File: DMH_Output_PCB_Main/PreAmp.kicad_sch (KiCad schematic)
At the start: 39 parts, among them J13 Conn_01x06, J28 Conn_01x06, U16 NE5532, U17 NE5532, U18 NE5532, U19 NE5532

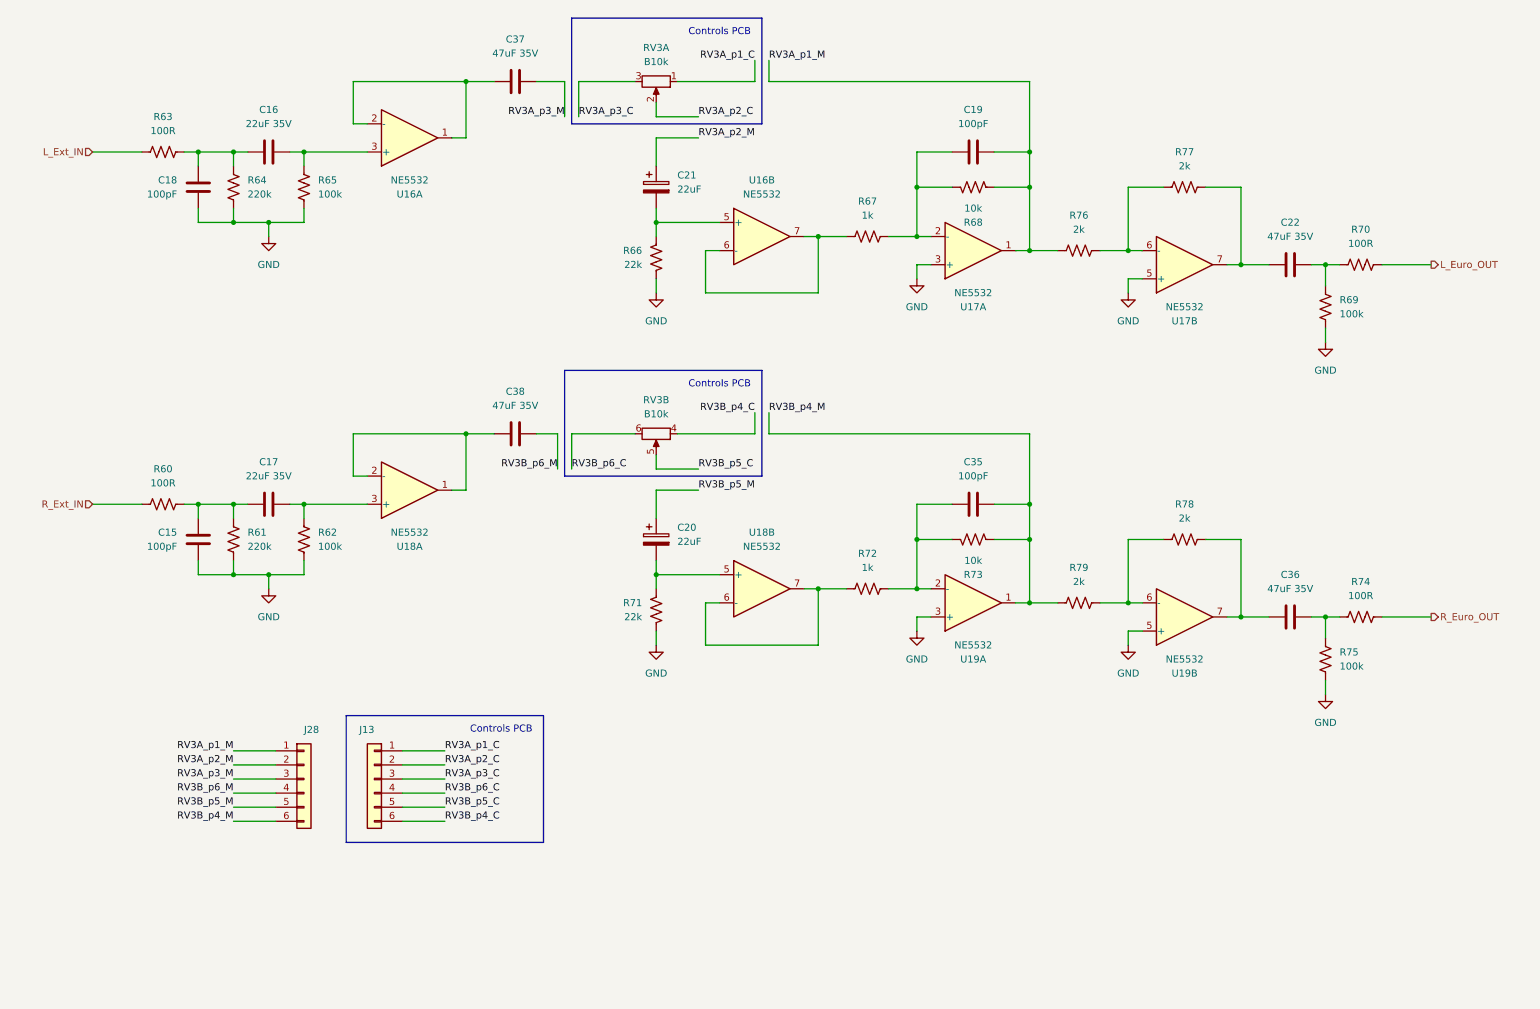
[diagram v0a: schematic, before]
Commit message: Prepped for Main PCB design
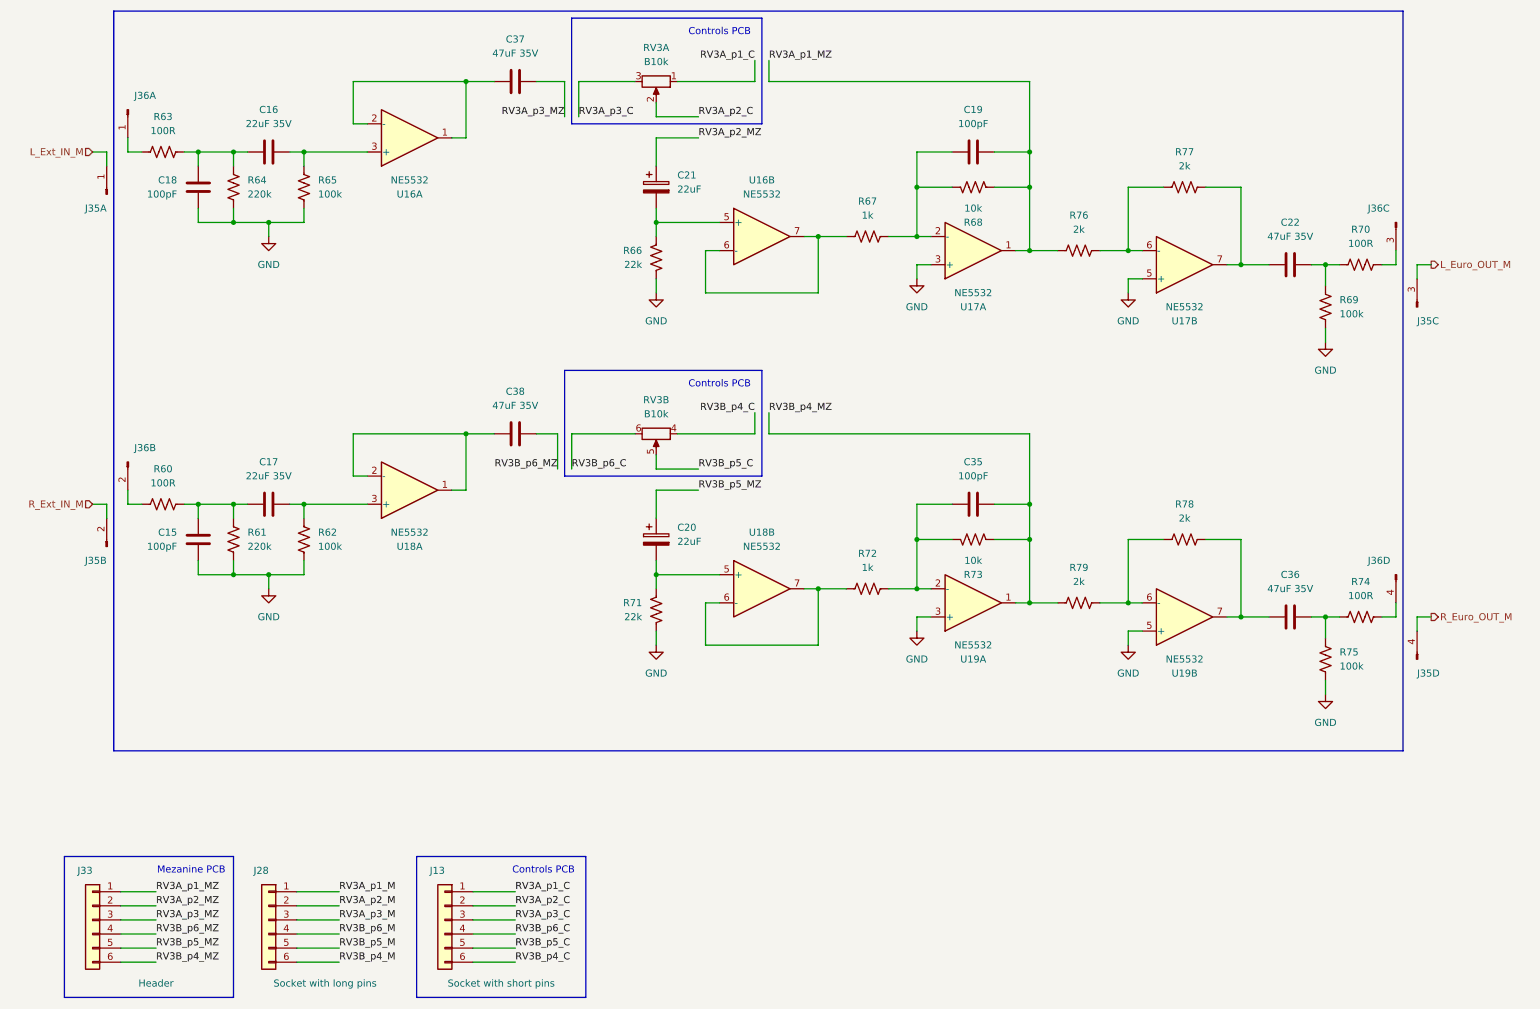
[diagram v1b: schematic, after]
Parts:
- added J33: Conn_01x06, Connector_PinHeader_2.54mm:PinHeader_1x06_P2.54mm_Vertical, symbol Connector_Generic:Conn_01x06
- added J35: Conn_01x04_PinHeader, Connector_PinSocket_2.54mm:PinSocket_1x04_P2.54mm_Vertical, symbol SynthStuff:Conn_01x04_PinHeader
- added J36: Conn_01x04_PinHeader, Connector_PinHeader_2.54mm:PinHeader_1x04_P2.54mm_Vertical, symbol SynthStuff:Conn_01x04_PinHeader
- J28: footprint Connector_PinHeader_2.54mm:PinHeader_1x06_P2.54mm_Vertical -> Connector_PinSocket_2.54mm:PinSocket_1x06_P2.54mm_Vertical
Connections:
- net RV3A_p1_M: no longer C19.2, R68.2, R76.1, U17.1
- net RV3A_p2_M: no longer C21.1
- net RV3A_p3_M: no longer C37.2
- net RV3B_p4_M: no longer C35.2, R73.2, R79.1, U19.1
- net RV3B_p5_M: no longer C20.1
- net RV3B_p6_M: no longer C38.2
- net L_Euro_OUT: no longer names the net of R70.2
- net L_Euro_OUT: now also J36.3 (Pin_3)
- net L_Ext_IN: no longer names the net of R63.1
- net L_Ext_IN: now also J36.1 (Pin_1)
- net R_Euro_OUT: no longer names the net of R74.2
- net R_Euro_OUT: now also J36.4 (Pin_4)
- net R_Ext_IN: no longer names the net of R60.1
- net R_Ext_IN: now also J36.2 (Pin_2)
- new net L_Euro_OUT_M: J35.3 (Pin_3)
- new net L_Ext_IN_M: J35.1 (Pin_1)
- new net RV3A_p1_MZ: C19.2, J33.1 (Pin_1), R68.2, R76.1, U17.1
- new net RV3A_p2_MZ: C21.1, J33.2 (Pin_2)
- new net RV3A_p3_MZ: C37.2, J33.3 (Pin_3)
- new net RV3B_p4_MZ: C35.2, J33.6 (Pin_6), R73.2, R79.1, U19.1
- new net RV3B_p5_MZ: C20.1, J33.5 (Pin_5)
- new net RV3B_p6_MZ: C38.2, J33.4 (Pin_4)
- new net R_Euro_OUT_M: J35.4 (Pin_4)
- new net R_Ext_IN_M: J35.2 (Pin_2)
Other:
- note added: "Mezanine PCB"
- moved on the sheet: J13, J28
